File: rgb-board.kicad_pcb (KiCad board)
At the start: 2 copper layers, 178 x 129.5 mm, 89 parts, among them J1 Conn_02x25_Odd_Even, J10 Conn_Coaxial, J11 Conn_Coaxial, J2 SCART-F, J3 TEST_1P, J4 TEST_1P, J5 Conn_Coaxial, J6 Conn_Coaxial, J7 Conn_Coaxial, J8 Conn_Coaxial, J9 Conn_Coaxial, Q101 BC550, Q105 BC550, Q109 BC550, Q113 BC550, Q114 BC550, Q201 BC550, SW1 SW_DPDT_x2, U1 LM2940-12

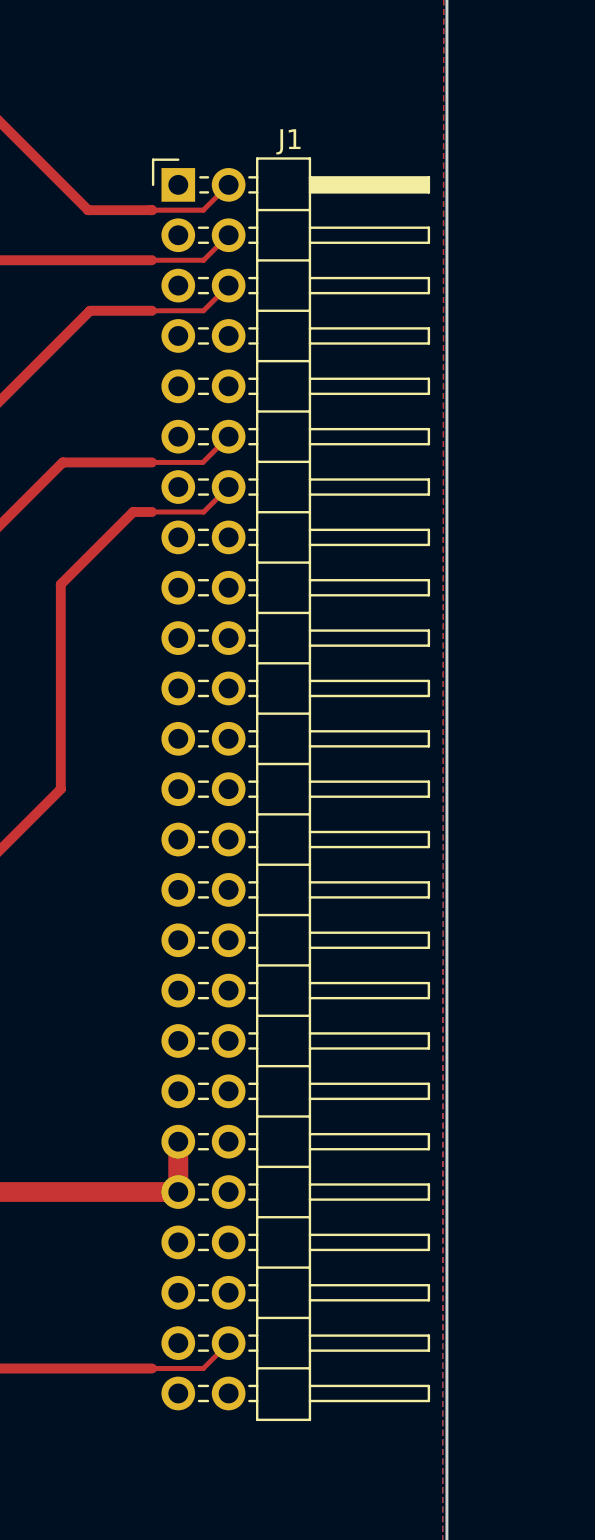
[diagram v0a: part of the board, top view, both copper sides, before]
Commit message: Moved around a bit
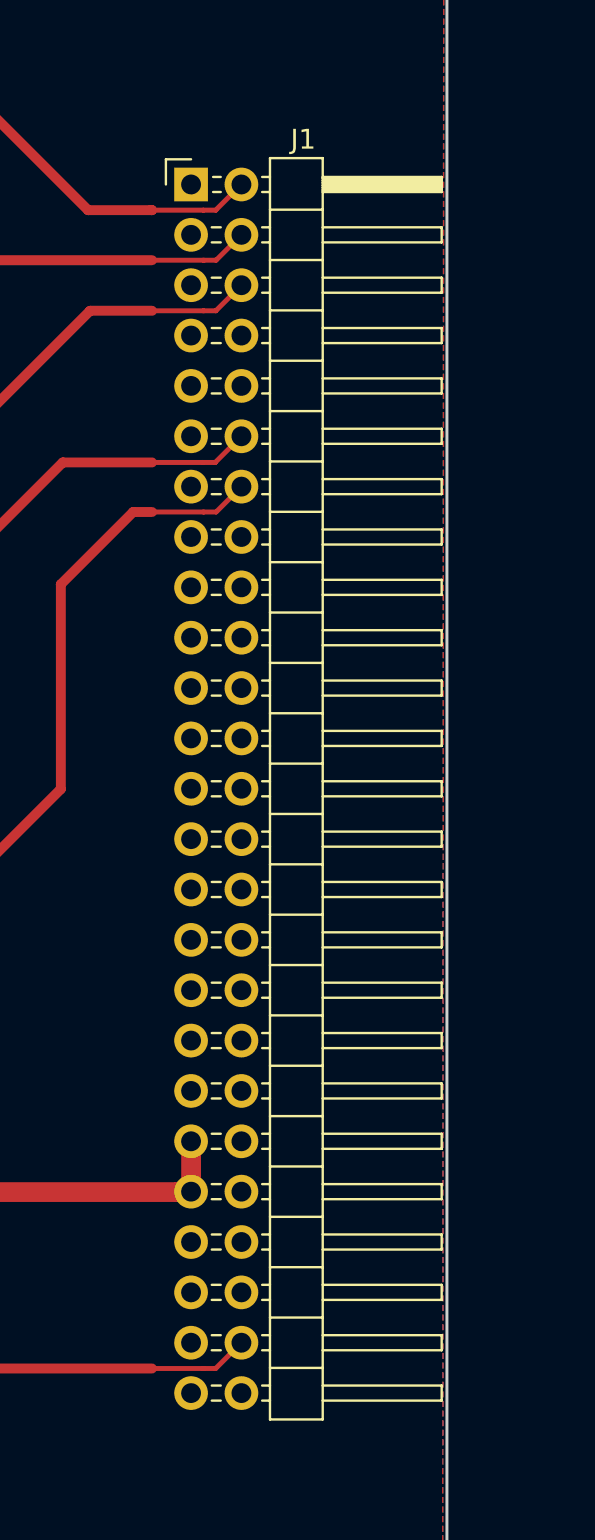
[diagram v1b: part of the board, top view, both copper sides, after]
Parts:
- moved J1 0.65 mm to (214.9, 64.6)
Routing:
- net /VCC+14V: track 85.0 -> 86.2 mm
- net /Y: track 101.8 -> 102.5 mm
- net /VD_: track 129.5 -> 130.1 mm
- net /R-Y: track 96.0 -> 96.6 mm
- net /HD: track 116.3 -> 116.9 mm
- net /B-Y: track 94.6 -> 95.3 mm
- net /AUDIO_: track 110.7 -> 111.4 mm
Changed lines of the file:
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@@
     (thickness 1.6)
     (drawings 58)
-    (tracks 312)
+    (tracks 321)
     (zones 0)
     (modules 89)
@@
   )
   (setup
-    (last_trace_width 1)
+    (last_trace_width 0.25)
     (user_trace_width 0.25)
     (user_trace_width 1)
@@
   )
   (module Pin_Headers:Pin_Header_Angled_2x25_Pitch2.54mm (layer F.Cu)
-    (at 214.275 64.65)
+    (at 214.92 64.63)
     (descr "Through hole angled pin header, 2x25, 2.54mm pitch, 6mm pin length, double rows")
     (tags "Through hole angled pin header THT 2x25 2.54mm double row")
@@
   (segment (start 151.905 134.88) (end 153.225 136.2) (width 1) (layer B.Cu) (net 8) (status 10))
   (segment (start 153.225 136.2) (end 153.225 139.1) (width 1) (layer B.Cu) (net 8) (status 20))
-  (segment (start 214.275 115.45) (end 214.275 112.785) (width 1) (layer F.Cu) (net 9))
+  (segment (start 214.92 115.43) (end 214.295 115.43) (width 1) (layer F.Cu) (net 9))
+  (segment (start 214.295 115.43) (end 214.275 115.45) (width 1) (layer F.Cu) (net 9))
+  (segment (start 214.275 115.45) (end 214.92 115.43) (width 1) (layer F.Cu) (net 9))
+  (segment (start 214.92 112.89) (end 214.92 115.43) (width 1) (layer F.Cu) (net 9))
   (segment (start 146.825 139.1) (end 147 139.1) (width 1) (layer F.Cu) (net 9))
   (segment (start 147 139.1) (end 149.7 136.4) (width 1) (layer F.Cu) (net 9))
@@
   (segment (start 109.575 141.73) (end 109.605 141.7) (width 0.5) (layer F.Cu) (net 11) (status 30))
   (segment (start 109.591 141.686) (end 109.605 141.7) (width 0.5) (layer F.Cu) (net 11) (status 30))
+  (segment (start 215.535 124.35) (end 216.16 124.35) (width 0.25) (layer F.Cu) (net 12))
+  (segment (start 216.16 124.35) (end 217.46 123.05) (width 0.25) (layer F.Cu) (net 12))
   (segment (start 212.95 124.35) (end 215.535 124.35) (width 0.25) (layer F.Cu) (net 12))
-  (segment (start 216.815 123.07) (end 215.535 124.35) (width 0.25) (layer F.Cu) (net 12))
   (segment (start 212.95 124.35) (end 202.55 124.35) (width 0.5) (layer F.Cu) (net 12))
   (segment (start 136.65 140.4) (end 131.425 140.4) (width 0.5) (layer F.Cu) (net 12))
@@
   (segment (start 131.425 140.4) (end 131.425 140.3) (width 0.5) (layer F.Cu) (net 12) (status 30))
   (segment (start 131.425 140.4) (end 131.625 140.4) (width 0.5) (layer F.Cu) (net 12) (status 30))
+  (segment (start 215.54 65.925) (end 216.165 65.925) (width 0.25) (layer F.Cu) (net 13))
+  (segment (start 216.165 65.925) (end 217.46 64.63) (width 0.25) (layer F.Cu) (net 13))
   (segment (start 212.95 65.925) (end 215.54 65.925) (width 0.25) (layer F.Cu) (net 13))
-  (segment (start 215.54 65.925) (end 216.815 64.65) (width 0.25) (layer F.Cu) (net 13))
   (segment (start 185.4 41.6) (end 209.725 65.925) (width 0.5) (layer F.Cu) (net 13))
   (segment (start 209.725 65.925) (end 212.95 65.925) (width 0.5) (layer F.Cu) (net 13))
   (segment (start 212.95 65.925) (end 212.9 65.925) (width 0.5) (layer F.Cu) (net 13))
   (segment (start 125.62 41.6) (end 185.4 41.6) (width 0.5) (layer F.Cu) (net 13))
+  (segment (start 215.555 68.45) (end 216.18 68.45) (width 0.25) (layer F.Cu) (net 14))
+  (segment (start 216.18 68.45) (end 217.46 67.17) (width 0.25) (layer F.Cu) (net 14))
   (segment (start 212.95 68.45) (end 215.555 68.45) (width 0.25) (layer F.Cu) (net 14))
-  (segment (start 216.815 67.19) (end 215.555 68.45) (width 0.25) (layer F.Cu) (net 14))
   (segment (start 179.5 61.4) (end 186.55 68.45) (width 0.5) (layer F.Cu) (net 14))
   (segment (start 186.55 68.45) (end 212.95 68.45) (width 0.5) (layer F.Cu) (net 14))
   (segment (start 179.5 61.4) (end 125.62 61.4) (width 0.5) (layer F.Cu) (net 14))
+  (segment (start 215.545 71) (end 216.17 71) (width 0.25) (layer F.Cu) (net 15))
+  (segment (start 216.17 71) (end 217.46 69.71) (width 0.25) (layer F.Cu) (net 15))
   (segment (start 212.95 71) (end 215.545 71) (width 0.25) (layer F.Cu) (net 15))
-  (segment (start 216.815 69.73) (end 215.545 71) (width 0.25) (layer F.Cu) (net 15))
   (segment (start 199.525 81.3) (end 209.825 71) (width 0.5) (layer F.Cu) (net 15))
   (segment (start 209.825 71) (end 212.95 71) (width 0.5) (layer F.Cu) (net 15))
   (segment (start 199.525 81.3) (end 125.62 81.3) (width 0.5) (layer F.Cu) (net 15))
+  (segment (start 215.515 78.65) (end 216.14 78.65) (width 0.25) (layer F.Cu) (net 16))
+  (segment (start 216.14 78.65) (end 217.46 77.33) (width 0.25) (layer F.Cu) (net 16))
   (segment (start 212.95 78.65) (end 215.515 78.65) (width 0.25) (layer F.Cu) (net 16))
-  (segment (start 216.815 77.35) (end 215.515 78.65) (width 0.25) (layer F.Cu) (net 16))
   (segment (start 130.41 100.09) (end 134.65 95.85) (width 0.5) (layer F.Cu) (net 16))
   (segment (start 134.65 95.85) (end 191.25 95.85) (width 0.5) (layer F.Cu) (net 16))
@@
   (segment (start 113.4 101.05) (end 113.4 100.09) (width 0.5) (layer F.Cu) (net 16) (status 20))
   (segment (start 112.9 101.55) (end 113.4 101.05) (width 0.5) (layer F.Cu) (net 16))
+  (segment (start 215.555 81.15) (end 216.18 81.15) (width 0.25) (layer F.Cu) (net 17))
+  (segment (start 216.18 81.15) (end 217.46 79.87) (width 0.25) (layer F.Cu) (net 17))
   (segment (start 212.95 81.15) (end 215.555 81.15) (width 0.25) (layer F.Cu) (net 17))
-  (segment (start 216.815 79.89) (end 215.555 81.15) (width 0.25) (layer F.Cu) (net 17))
   (segment (start 128.41 120.04) (end 113.4 120.04) (width 0.5) (layer F.Cu) (net 17))
   (segment (start 208.35 84.8) (end 212 81.15) (width 0.5) (layer F.Cu) (net 17))
